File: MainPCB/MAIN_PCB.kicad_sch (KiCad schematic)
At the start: 43 parts, among them U1 INA226, U2 DRV8871DDA, U3 INA226

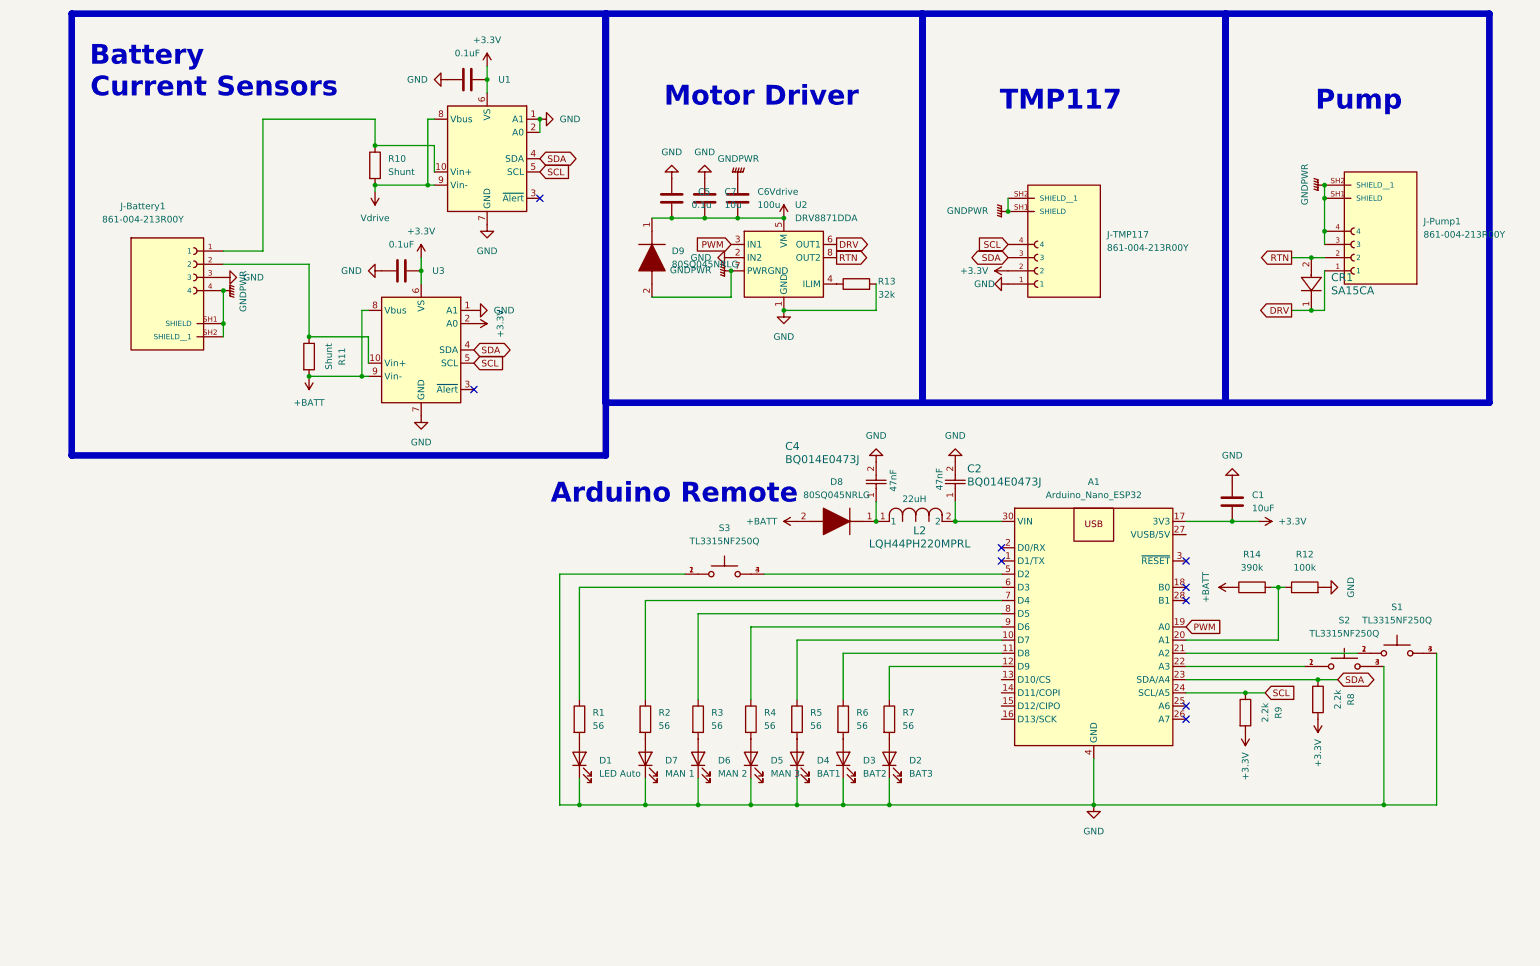
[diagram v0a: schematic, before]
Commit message: hella changes
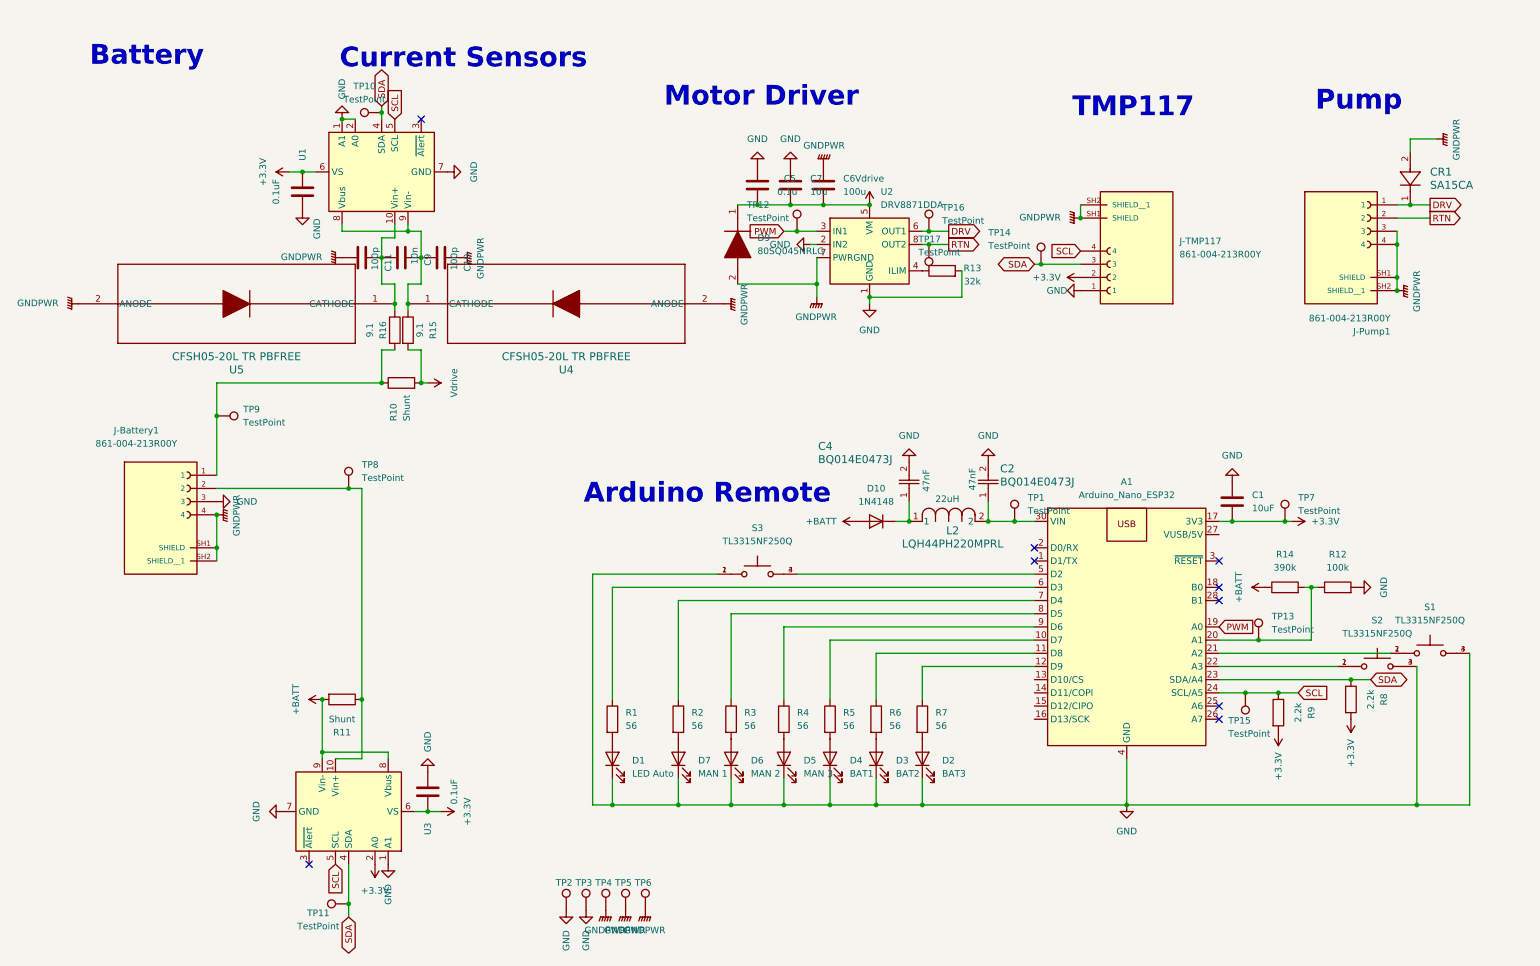
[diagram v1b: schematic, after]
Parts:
- removed D8: 80SQ045NRLG, 80SQ045NRLG:DIOAD2860W130L840D505, symbol 80SQ045NRLG:80SQ045NRLG
- added C10, C11: 100p, CAP_BF01:CAP_BF01_AVX, symbol Device:C
- added C9: 10n, CAP_BF01:CAP_BF01_AVX, symbol Device:C
- added D10: 1N4148, Diode_THT:D_DO-35_SOD27_P7.62mm_Horizontal, symbol Diode:1N4148
- added R15, R16: 9.1, Resistor_THT:R_Axial_DIN0207_L6.3mm_D2.5mm_P10.16mm_Horizontal, symbol Device:R
- added TP1, TP10, TP11, TP12, TP13, TP14, TP15, TP16, TP17, TP2, TP3, TP4, TP5, TP6, TP7, TP8, TP9: TestPoint, TestPoint:TestPoint_THTPad_D1.5mm_Drill0.7mm, symbol Connector:TestPoint
- added U4, U5: CFSH05-20L TR PBFREE, Shotky:CFSH05-20L TR PBFREE_CNS, symbol 2026-03-11_05-59-29:CFSH05-20L_TR_PBFREE
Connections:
- net +3.3V: now also TP7.1
- net +BATT: now also D10.2 (A)
- net DRV: now also TP16.1
- net GND: now also TP2.1, TP3.1; no longer U2.7 (GND)
- net GNDPWR: now also CR1.2, C10.1, C11.2, TP4.1, TP5.1, TP6.1, U4.2 (ANODE), U5.2 (ANODE)
- net PWM: now also TP12.1
- net RTN: now also TP17.1; no longer CR1.2
- net SCL: now also TP15.1
- net SDA: now also TP10.1, TP11.1, TP14.1
- net Vdrive: now also R15.2; no longer U1.8 (Vbus), U1.9 (Vin-)
- net at A1.20 (A1), R12.1, R14.2: now also TP13.1
- net at A1.30 (VIN), C2.1, L2.2: now also TP1.1
- net at J-Battery1.1, R10.1: now also R16.2, TP9.1; no longer U1.10 (Vin+)
- net at J-Battery1.2, R11.1, U3.10 (Vin+): now also TP8.1
- net at C4.1, L2.1: now also D10.1 (K)
- new net: C11.1, C9.2, R16.1, U1.10 (Vin+), U5.1 (CATHODE)
- new net: C10.2, C9.1, R15.1, U1.8 (Vbus), U1.9 (Vin-), U4.1 (CATHODE)
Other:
- moved on the sheet: A1, C2, C4, C5, C6, C7, CR1, D1, D2, D3, D4, D5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
